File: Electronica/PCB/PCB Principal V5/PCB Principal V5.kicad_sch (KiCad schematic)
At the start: 17 parts, among them J1 Conexion Sensores, J12 TP, J2 Power Monster, J3 On/Off General, J4 Power Input 2, J5 IDC Placa Botones, J6 Power Input 1, SW1 On/Off Motores

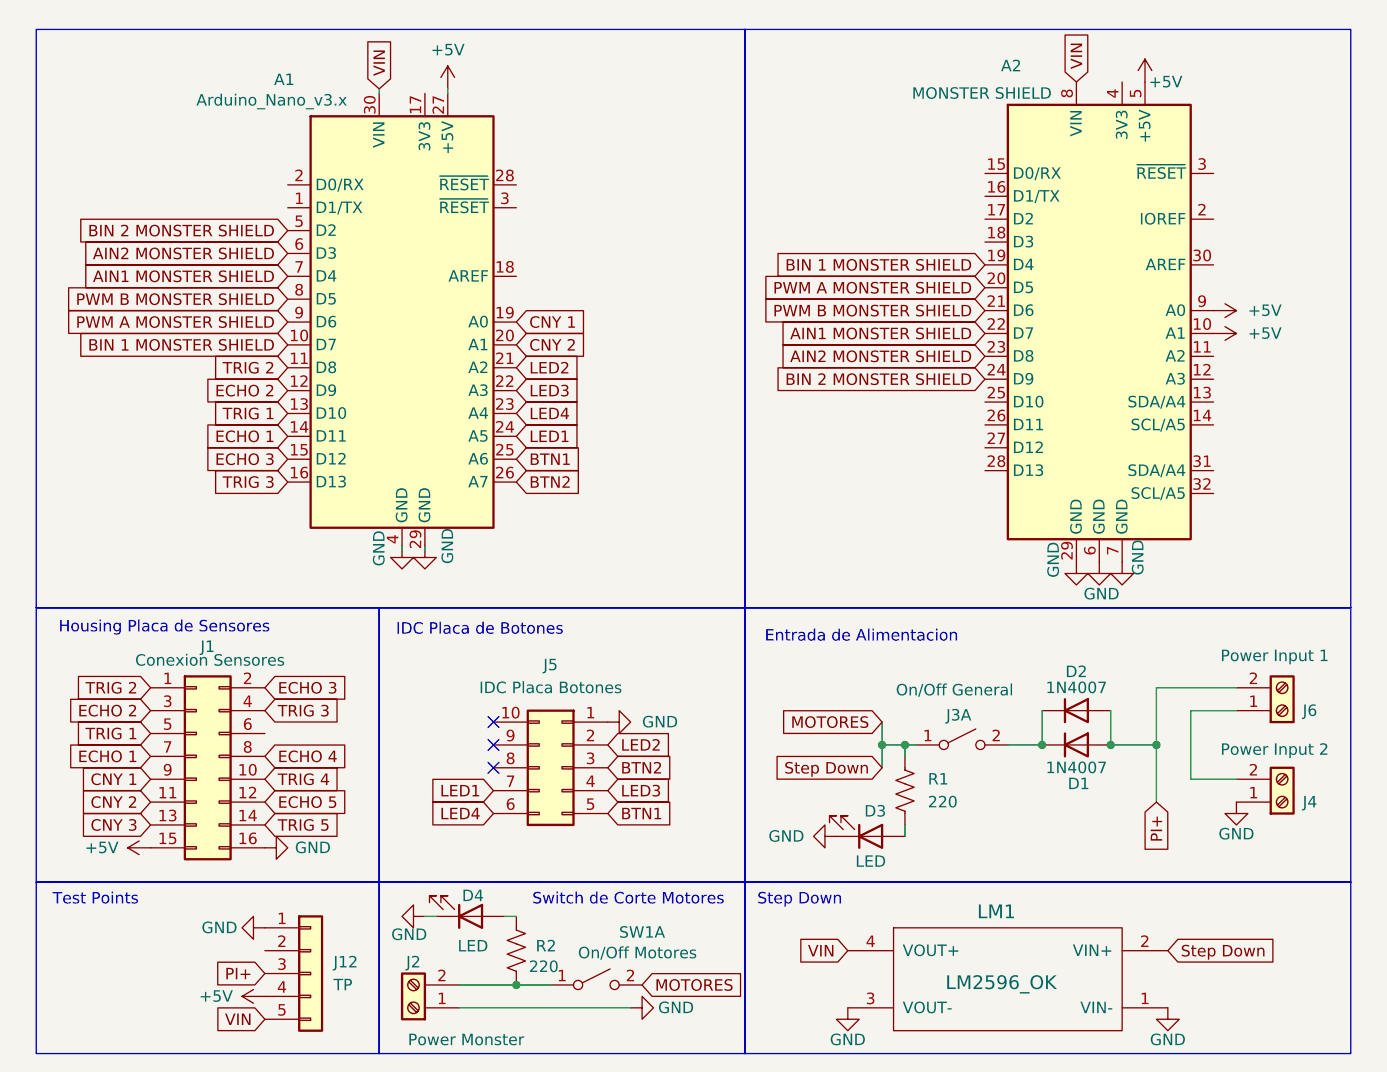
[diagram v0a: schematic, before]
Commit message: nada
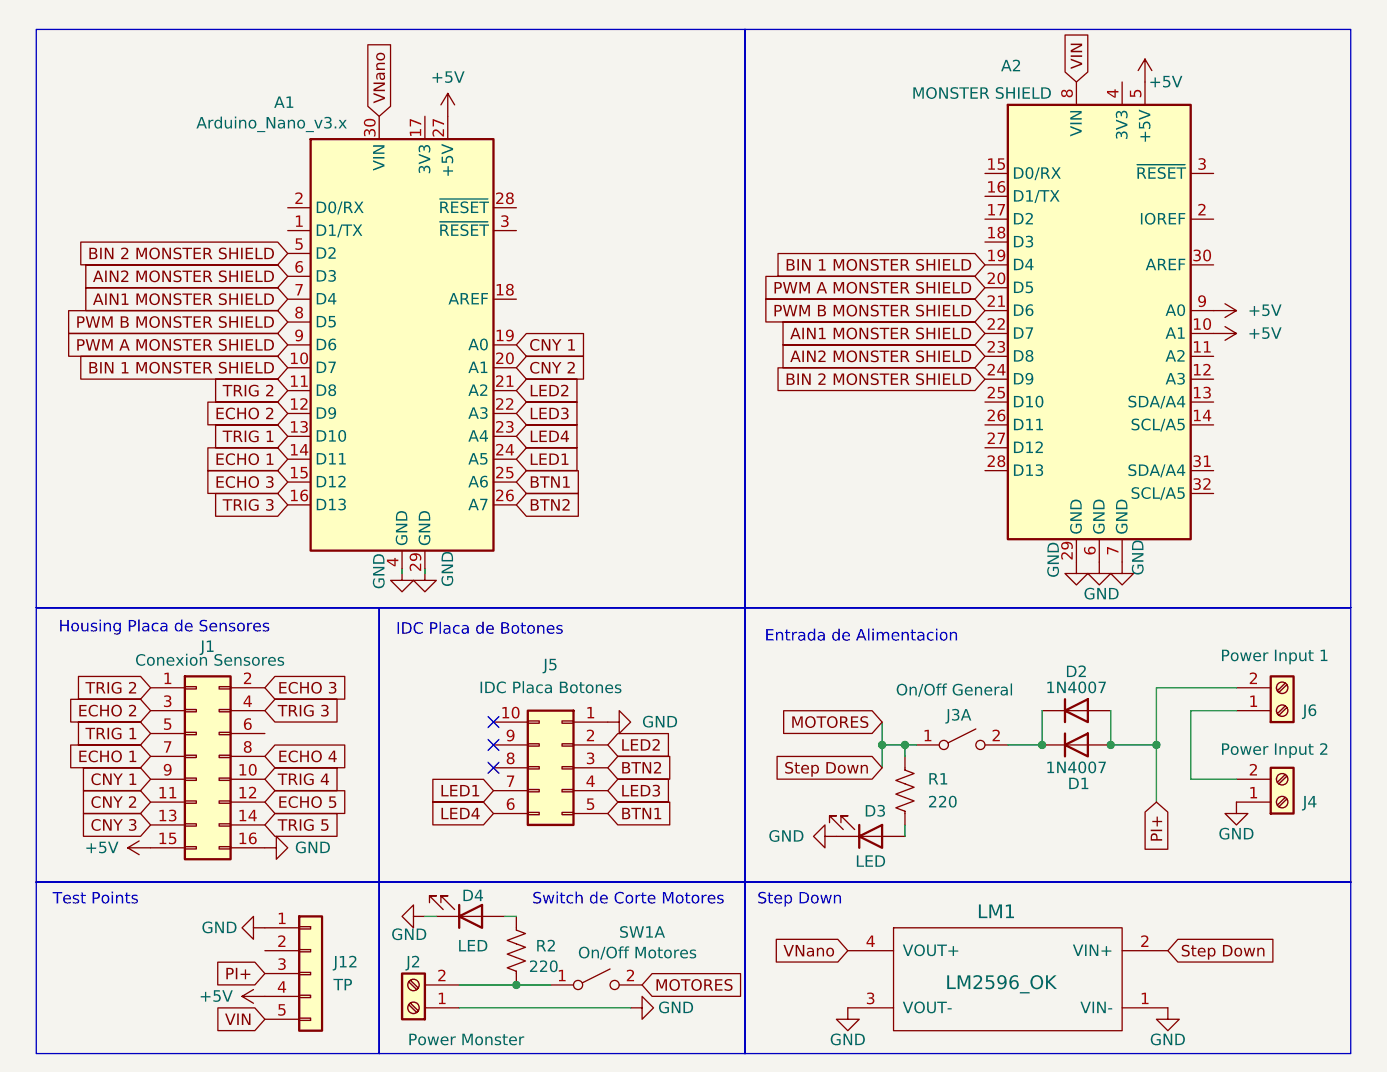
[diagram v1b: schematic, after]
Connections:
- net VIN: no longer A1.30 (VIN), LM1.4 (VOUT+)
- new net VNano: A1.30 (VIN), LM1.4 (VOUT+)
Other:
- moved on the sheet: A1

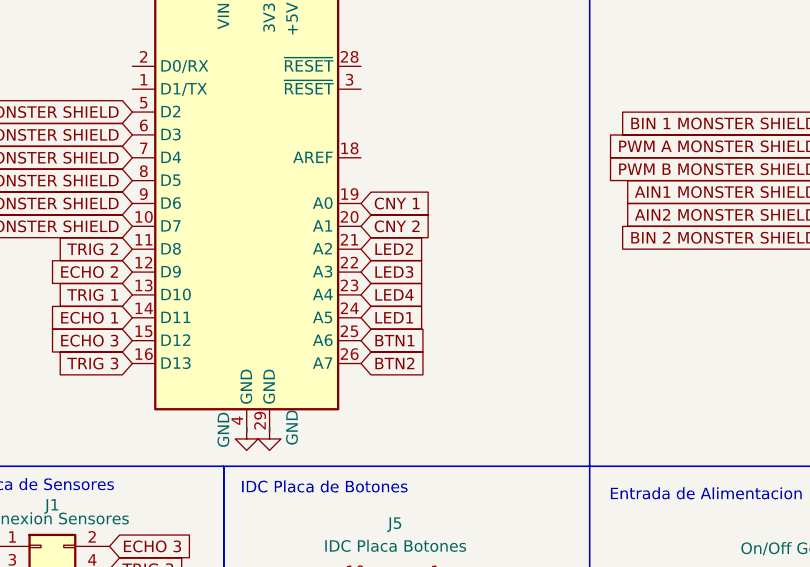
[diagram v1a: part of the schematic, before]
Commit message: .
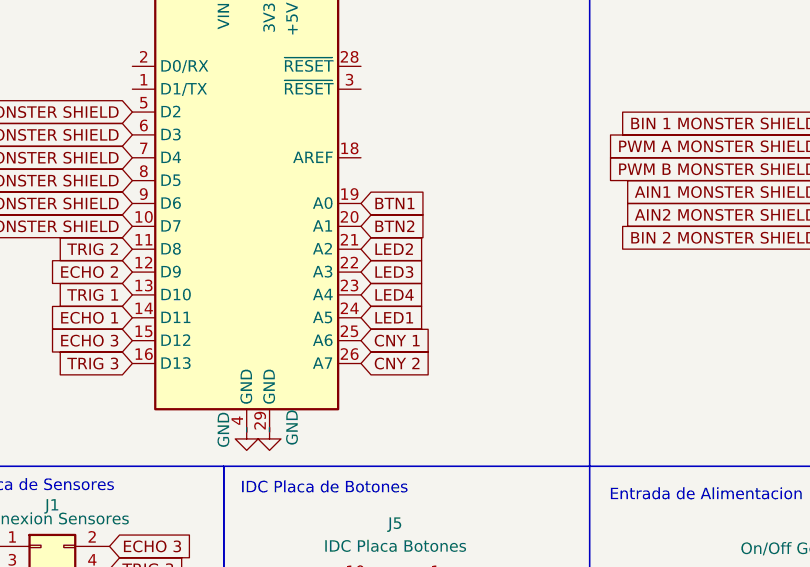
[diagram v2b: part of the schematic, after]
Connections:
- net BTN1: now also A1.19 (A0); no longer A1.25 (A6)
- net BTN2: now also A1.20 (A1); no longer A1.26 (A7)
- net CNY 1: now also A1.25 (A6); no longer A1.19 (A0)
- net CNY 2: now also A1.26 (A7); no longer A1.20 (A1)

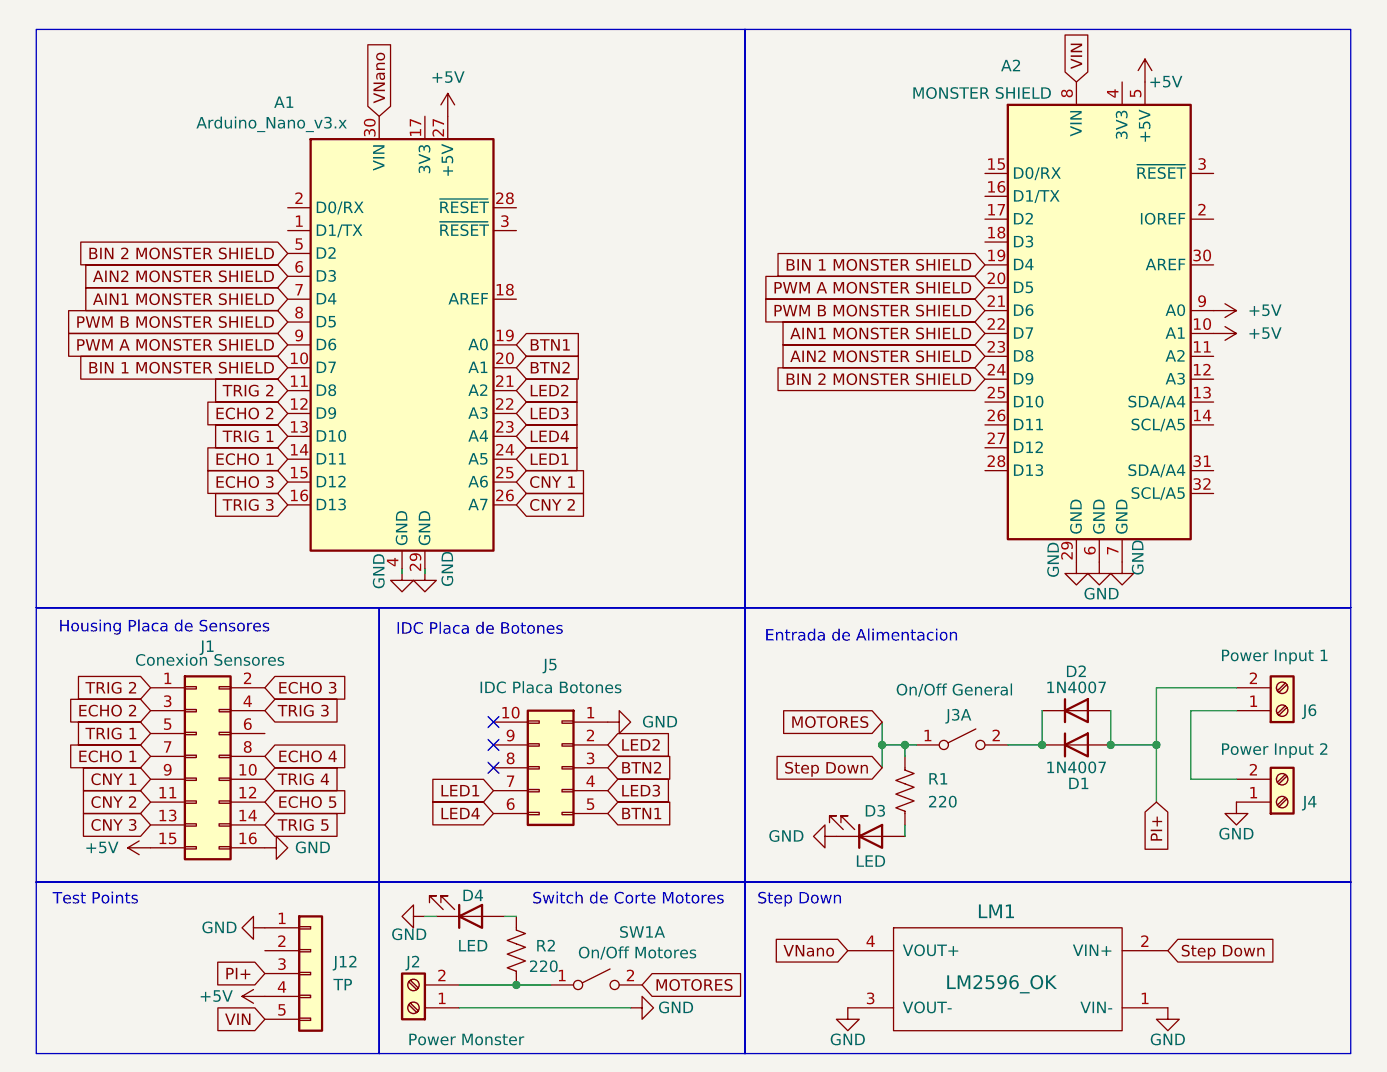
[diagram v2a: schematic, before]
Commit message: ,
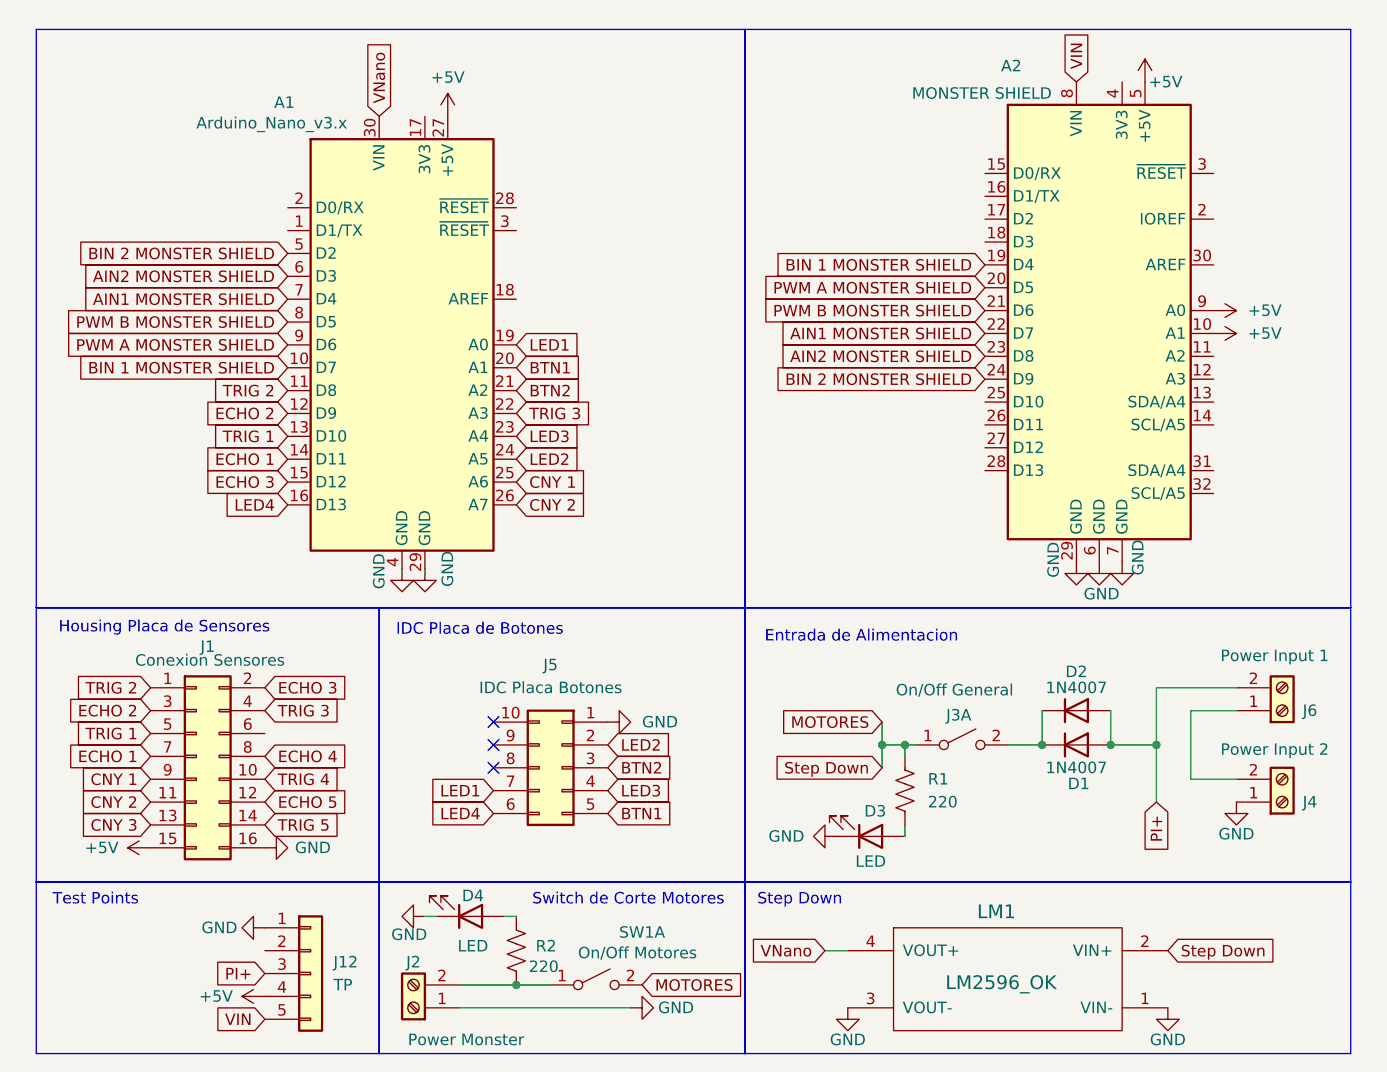
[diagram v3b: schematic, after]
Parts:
- LM1: footprint LM2596:LM2596_correctedMeas -> Step Down:LM2596_correctedMeas
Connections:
- net BTN1: now also A1.20 (A1); no longer A1.19 (A0)
- net BTN2: now also A1.21 (A2); no longer A1.20 (A1)
- net LED1: now also A1.19 (A0); no longer A1.24 (A5)
- net LED2: now also A1.24 (A5); no longer A1.21 (A2)
- net LED3: now also A1.23 (A4); no longer A1.22 (A3)
- net LED4: now also A1.16 (D13); no longer A1.23 (A4)
- net TRIG 3: now also A1.22 (A3); no longer A1.16 (D13)
